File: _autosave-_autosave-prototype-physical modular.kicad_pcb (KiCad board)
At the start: 2 copper layers, 100 x 164 mm, 183 parts, among them CON1 BARREL_JACK, CON2 SD_Card_SEEEDOPL, IC1 ATMEGA2560-A, P1 POWER, P10 PC, P11 CONN_UART, P12 PJ, P15 PH, P16 PF, P18 3VI2C, P19 PIGPIO, P20 MIDI_IN, P21 MIDI_OUT, P22 BUSTI, P23 BUSTO, P3 SPI, P7 PA, Q1 BSS138, Q2 BSS138, Q3 BSS138, Q4 BSS138, Q5 BSS138, Q6 BSS138, SW1 SW_PUSH, SW10 SW_PUSH, SW11 SW_PUSH, SW12 SW_PUSH, SW13 SW_PUSH, SW14 SW_PUSH, SW2 ROTARY_ENCODER_SWITCH, SW3 SW_PUSH, SW4 SW_PUSH, SW5 SW_PUSH, SW6 SW_PUSH, SW7 SW_PUSH, SW8 SW_PUSH, SW9 SW_PUSH, U1 NCP1117ST50T3G, U2 6N138, Y1 16MHz

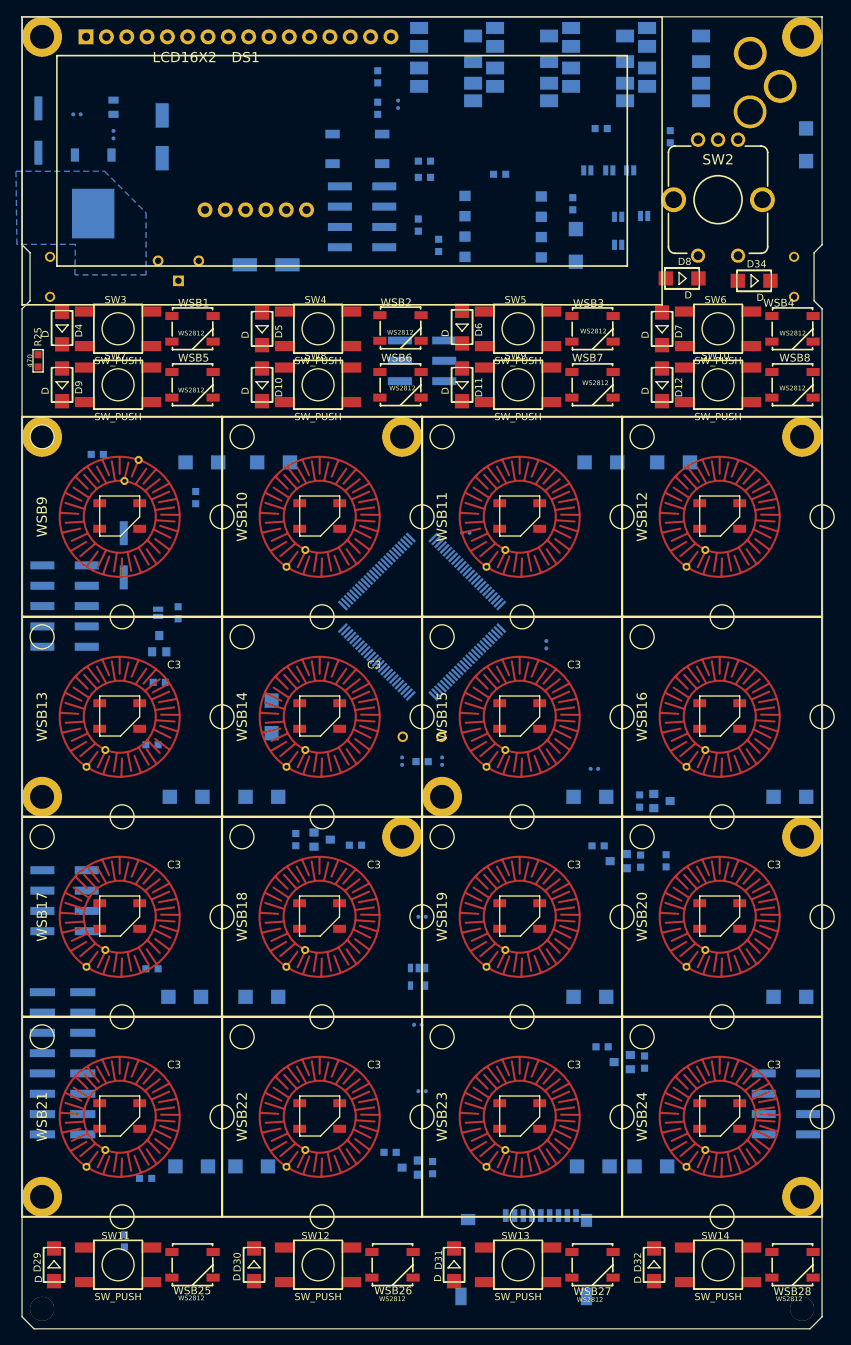
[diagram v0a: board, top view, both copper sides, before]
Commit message: new go at routing
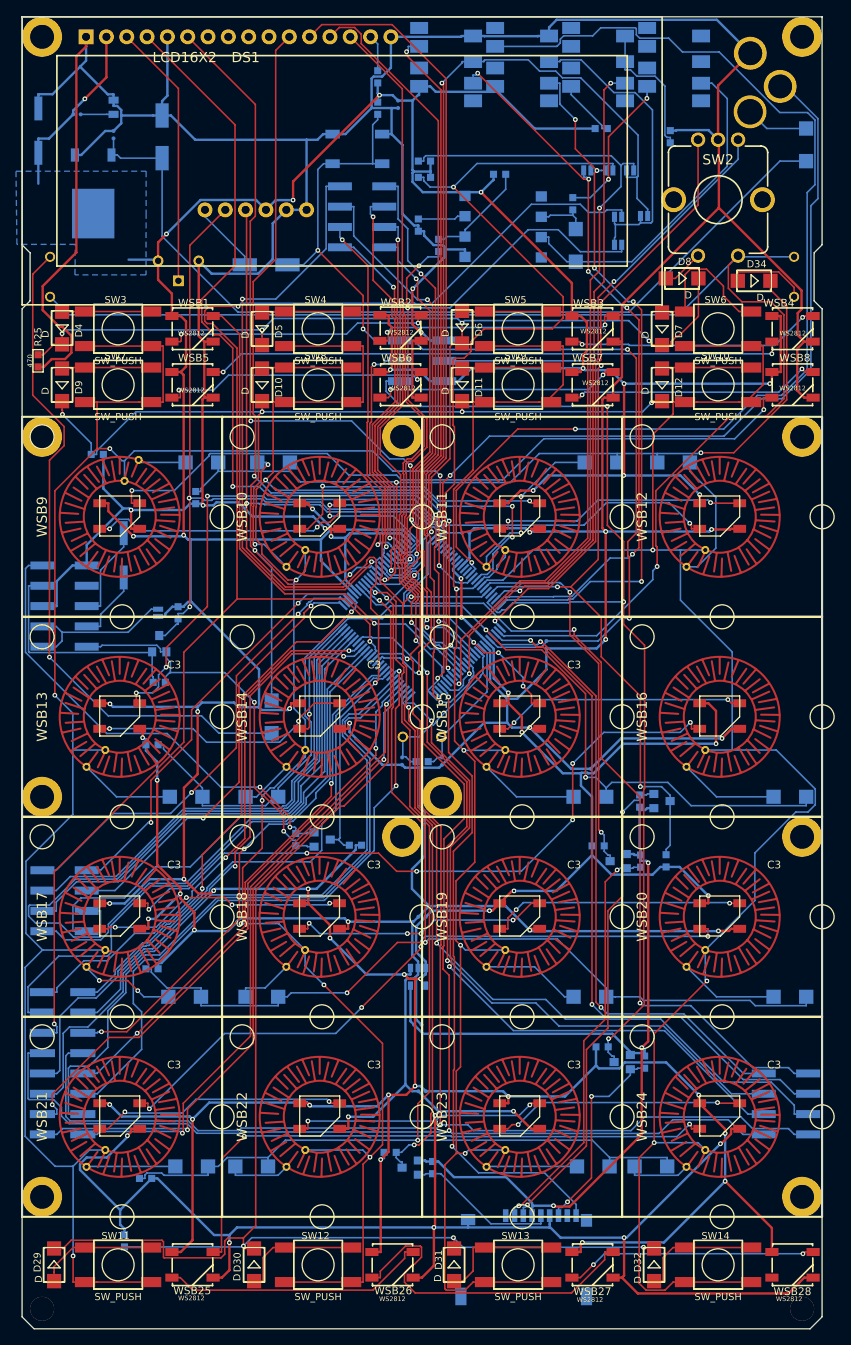
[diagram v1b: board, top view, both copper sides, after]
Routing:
- net GND: track 0.00 -> 995.8 mm, vias 0 -> 29
- net +5V: track 0.00 -> 813.9 mm, vias 0 -> 44
- net /BUS_COM: track 0.00 -> 289.4 mm, vias 0 -> 3
- net /TX3: track 0.00 -> 251.4 mm, vias 0 -> 3
- net /MUXAX0: track 0.00 -> 238.7 mm, vias 0 -> 5
- net /MUXAX1: track 0.00 -> 223.4 mm, vias 0 -> 8
- net /MUXAX3: track 0.00 -> 213.7 mm, vias 0 -> 3
- net /MUXBX6: track 0.00 -> 190.4 mm, vias 0 -> 4
- net Net-(IC1-Pad65): track 0.00 -> 185.4 mm, vias 0 -> 3
- net /MUXAX2: track 0.00 -> 182.6 mm, vias 0 -> 4
- net /MUXAX4: track 0.00 -> 175.1 mm, vias 0 -> 1
- net /MUXBX5: track 0.00 -> 148.0 mm, vias 0 -> 2
- net /MUXBX4: track 0.00 -> 143.8 mm, vias 0 -> 3
- net /MUXBX1: track 0.00 -> 141.2 mm, vias 0 -> 6
- net /BUSTO_CONN: track 0.00 -> 140.0 mm, vias 0 -> 2
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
